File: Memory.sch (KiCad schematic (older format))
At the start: 26 parts, among them U10 74LS05, U11 74HCT00, U12 74LS27, U13 74HC74, U14 74HC86, U2 AS6C4008-55PCN, U3 AS6C4008-55PCN, U4 AS6C4008-55PCN, U5 AS6C4008-55PCN, U6 74HCT00, U7 74LS32, U8 74LS32, U9 74LS05

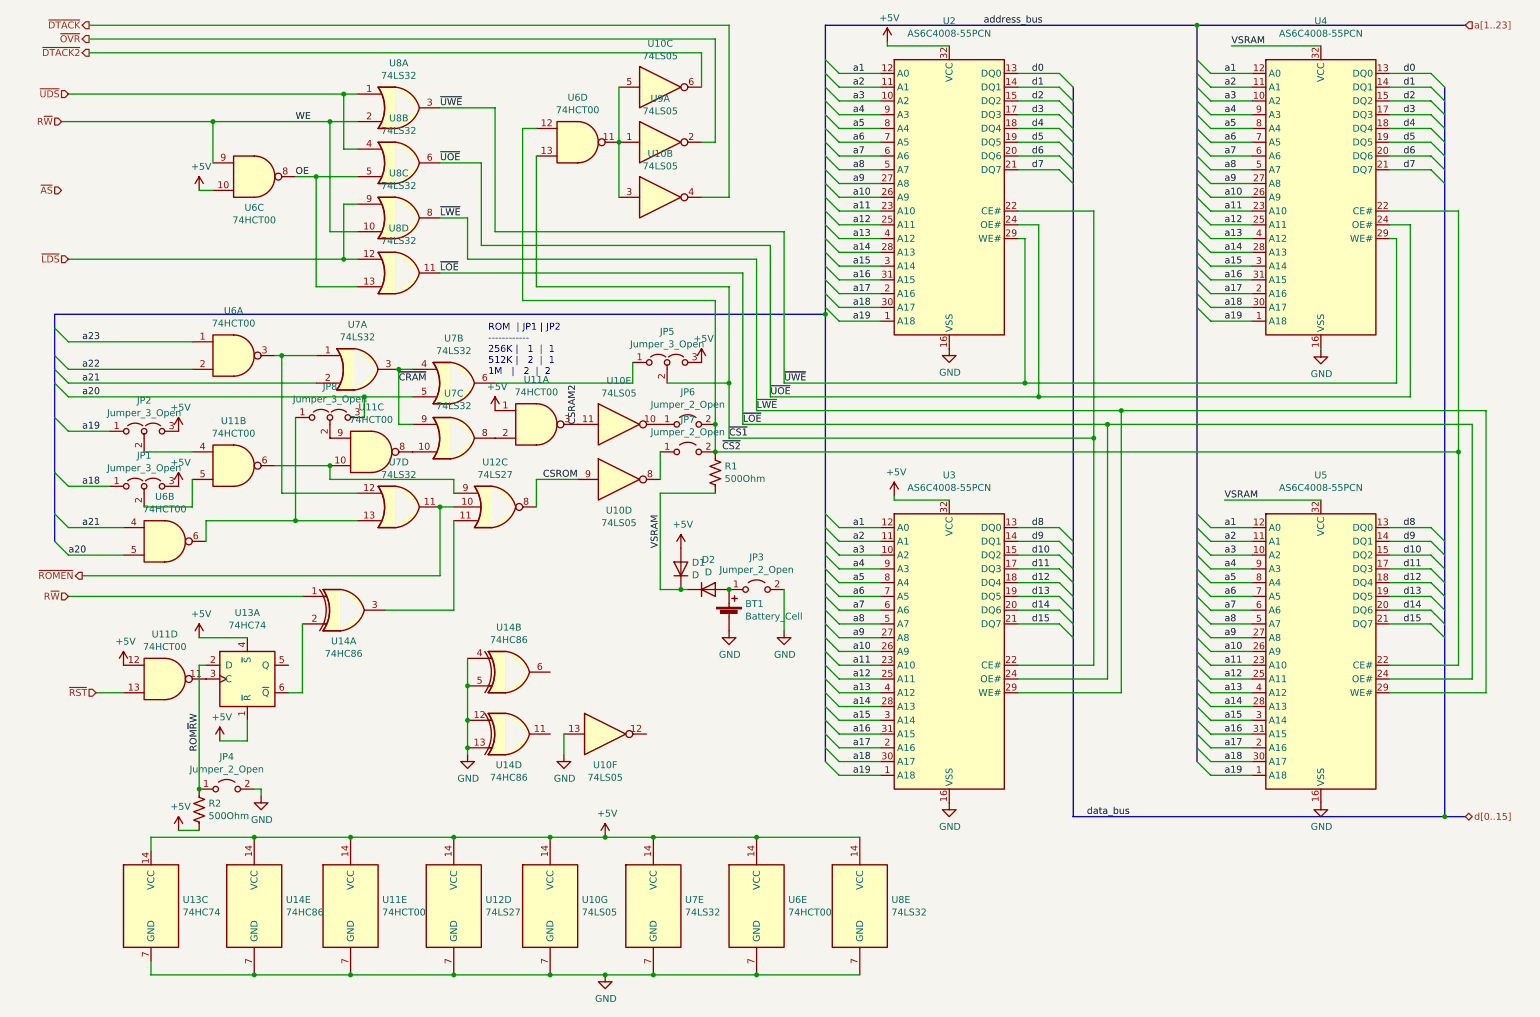
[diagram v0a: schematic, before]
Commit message: cleaning up a bit more
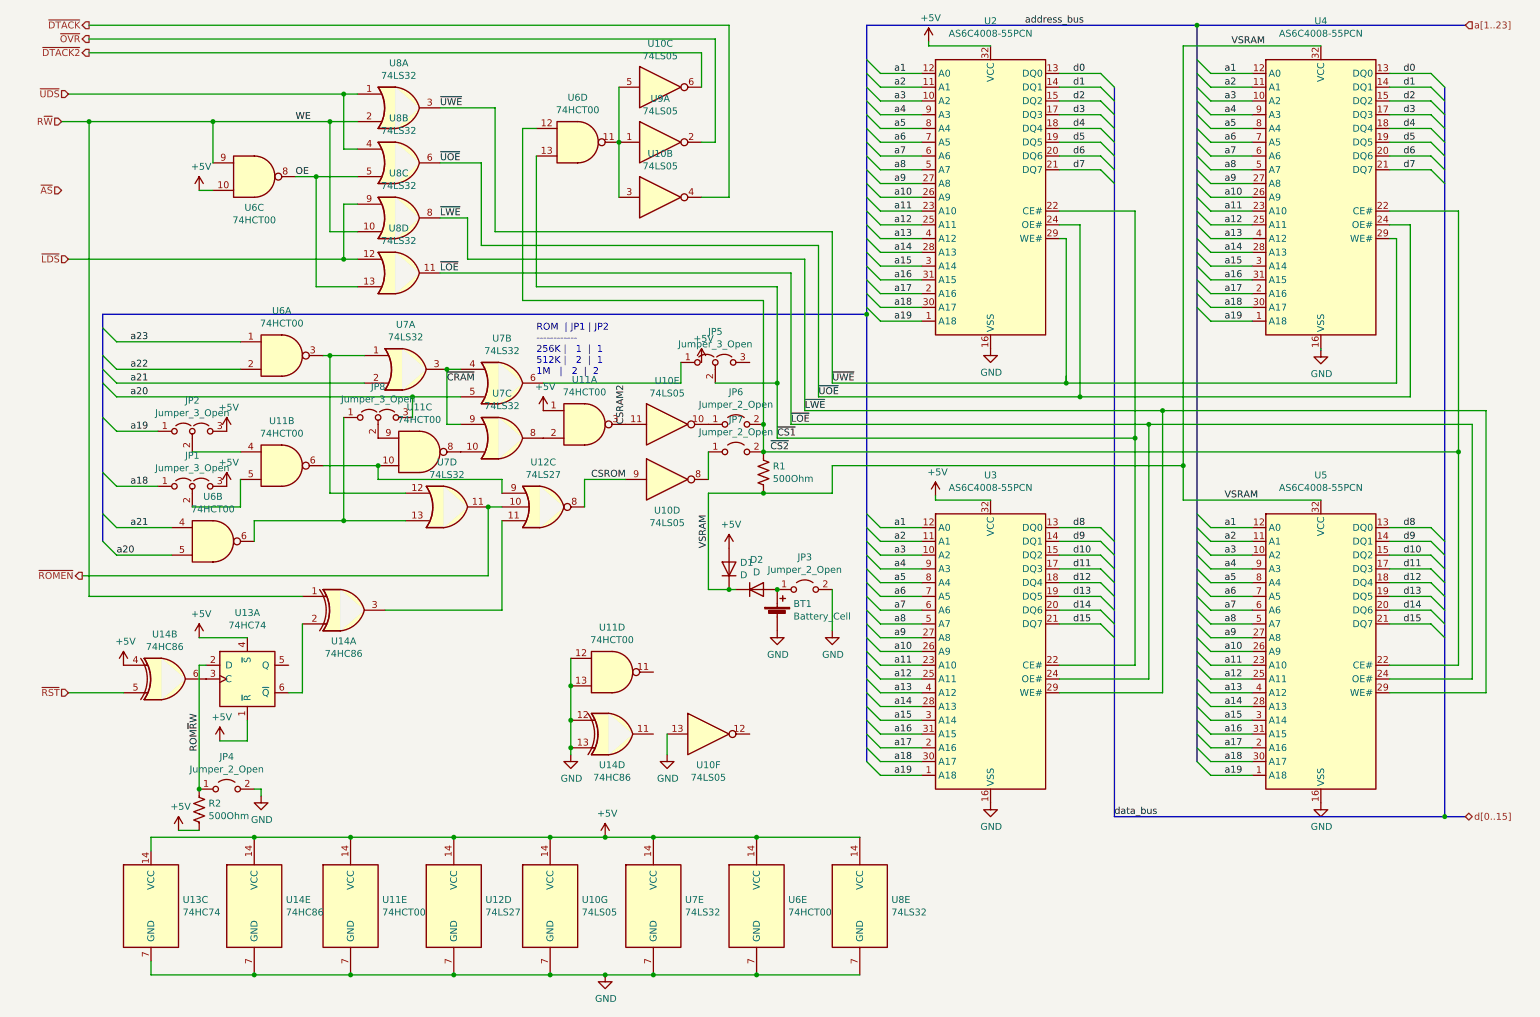
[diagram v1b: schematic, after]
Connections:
- net +5V: now also U14.4; no longer JP5.3 (B), U11.12
- net GND: now also U11.12, U11.13; no longer U14.4, U14.5
- net ~RST: now also U14.5; no longer U11.13
- net at U14.6: now also U13.3 (C)
- net at U11.11: no longer U13.3 (C)
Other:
- moved on the sheet: BT1, D1, D2, JP1, JP2, JP3, JP5, JP6, JP7, JP8, R1, U10D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
